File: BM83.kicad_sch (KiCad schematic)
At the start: 41 parts, among them J101 Jack-DC, J102 AudioJack3, J103 USB_C_Receptacle_USB2.0, J104 Conn_01x02, J105 Conn_01x02, SW101 SW_Slide_DPDT, U101 USBLC6-2SC6, U102 CH221K

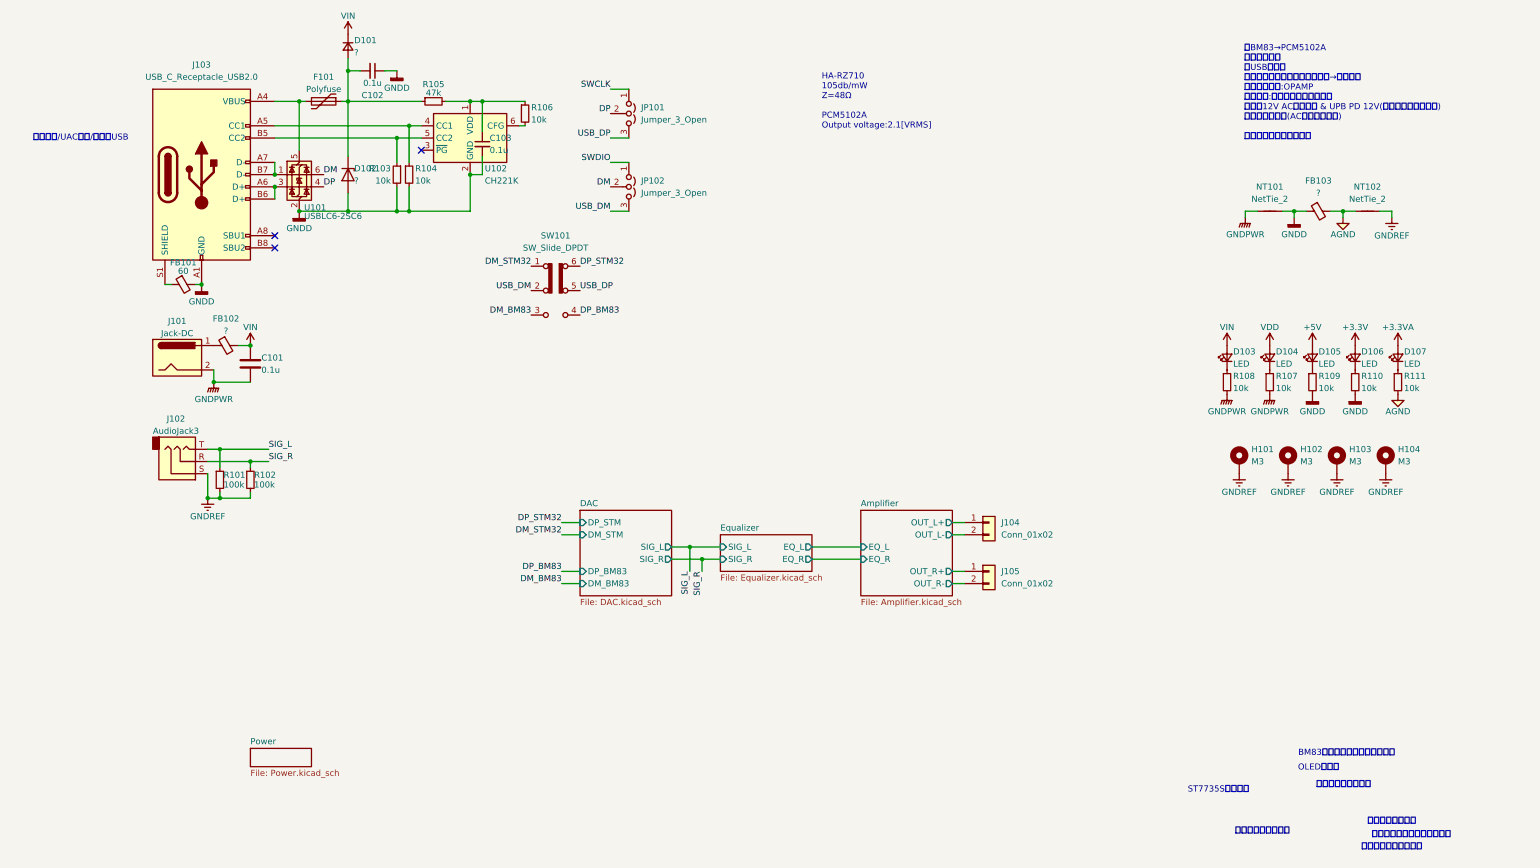
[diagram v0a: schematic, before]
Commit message: 回路図ひとまず完成
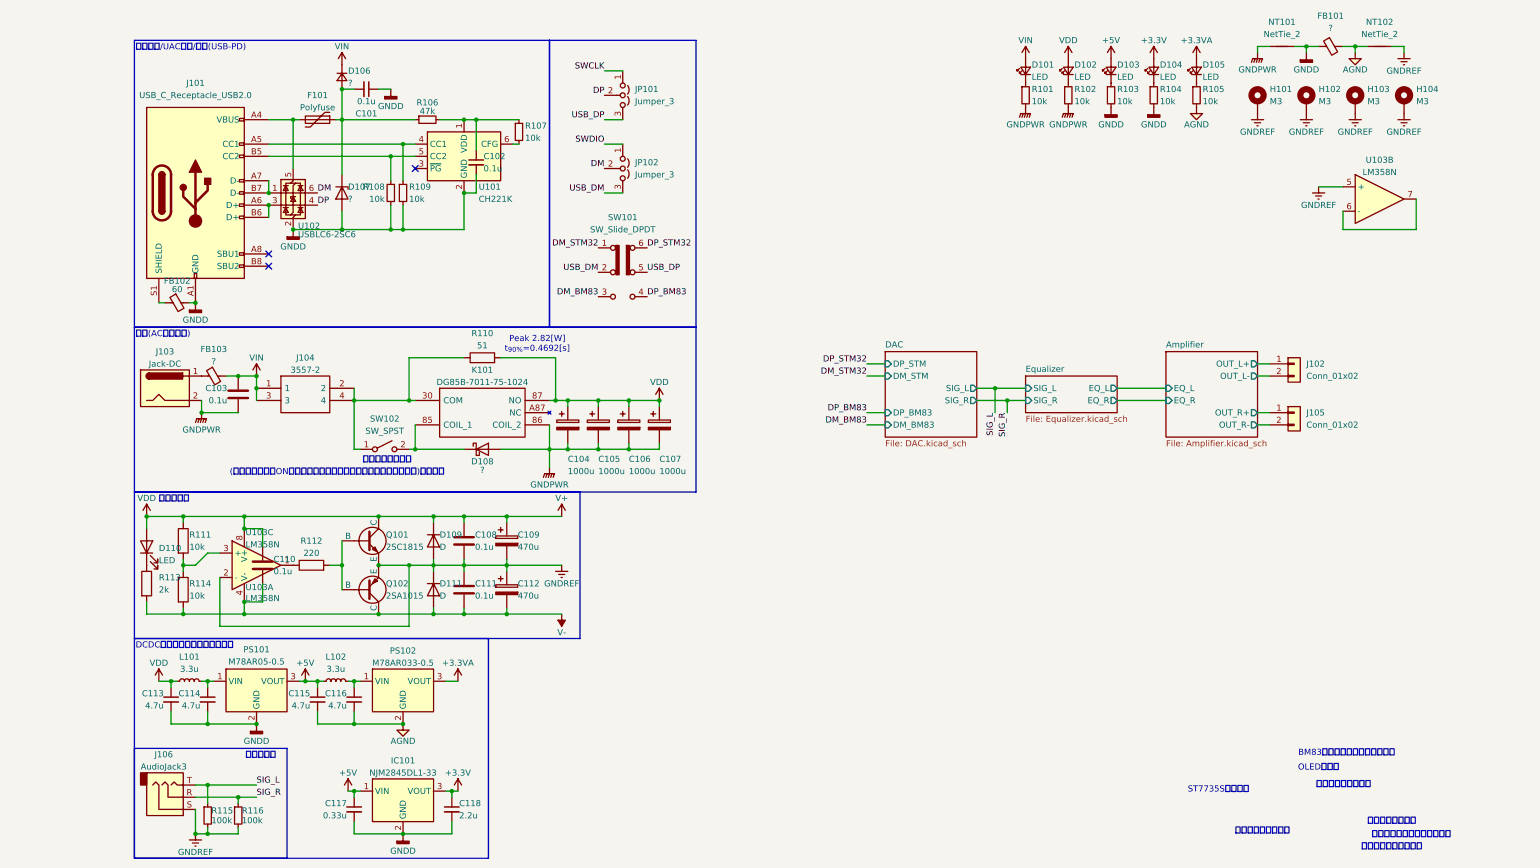
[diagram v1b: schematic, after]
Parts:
- added C104, C105, C106, C107: 1000u, Capacitor_THT:CP_Radial_D16.0mm_P7.50mm, symbol Device:C_Polarized
- added C108, C111: 0.1u, symbol Device:C
- added C109, C112: 470u, Capacitor_THT:CP_Radial_D16.0mm_P7.50mm, symbol Device:C_Polarized
- added C110: 0.1u, Capacitor_THT:C_Disc_D5.1mm_W3.2mm_P5.00mm, symbol Device:C
- added C113, C114, C115, C116: 4.7u, symbol Device:C_Small
- added C117: 0.33u, symbol Device:C_Small
- added C118: 2.2u, symbol Device:C_Small
- added D108: ?, samacsys:CUHS20F30H3F, symbol Device:D_Schottky
- added D109, D111: D, Diode_THT:D_DO-35_SOD27_P7.62mm_Horizontal, symbol Device:D
- added D110: LED, LED_THT:LED_D3.0mm_Horizontal_O1.27mm_Z2.0mm, symbol Device:LED
- added IC101: NJM2845DL1-33, TO-252-3-L1, symbol SamacSys_Parts:NJM2845DL1-33-TE1
- added J104: 3557-2, samacsys:3557-2, symbol SamacSys_Parts:3557-2
- added K101: DG85B-7011-75-1024, MyLibrary:DG85B-7011-75-1024, symbol SamaSys_Parts:DG85B-7011-75-1024
- added L101, L102: 3.3u, symbol Device:L_Small
- added PS101: M78AR05-0.5, M78AR03305, symbol SamacSys_Parts:M78AR05-0.5
- added PS102: M78AR033-0.5, M78AR03305, symbol SamacSys_Parts:M78AR033-0.5
- added Q101: 2SC1815, Package_TO_SOT_THT:TO-92L_Inline_Wide, symbol Simulation_SPICE:NPN
- added Q102: 2SA1015, Package_TO_SOT_THT:TO-92L_Inline_Wide, symbol Simulation_SPICE:PNP
- added R110: 51, symbol Device:R
- added R111, R114: 10k, Resistor_THT:R_Axial_DIN0204_L3.6mm_D1.6mm_P5.08mm_Horizontal, symbol Device:R
- added R112: 220, Resistor_THT:R_Axial_DIN0204_L3.6mm_D1.6mm_P5.08mm_Horizontal, symbol Device:R
- added R113: 2k, Resistor_THT:R_Axial_DIN0204_L3.6mm_D1.6mm_P5.08mm_Horizontal, symbol Device:R
- added SW102: SW_SPST, symbol Switch:SW_SPST
- added U103: LM358N, Package_DIP:DIP-8_W7.62mm_Socket, symbol Device:Opamp_Dual
- JP101, JP102: value Jumper_3_Open -> Jumper_3
- renumbered C102 to C101, C103 to C102, C101 to C103, D103 to D101, D104 to D102, D105 to D103, D106 to D104, D107 to D105, D101 to D106, D102 to D107, FB103 to FB101, FB101 to FB102, FB102 to FB103, J103 to J101, J104 to J102, J101 to J103, J102 to J106, R108 to R101, R107 to R102, R109 to R103, R110 to R104, R111 to R105, R105 to R106, R106 to R107, R103 to R108, R104 to R109, R101 to R115, R102 to R116, U102 to U101, U101 to U102
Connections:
- net +3.3V: now also C118.1, IC101.3 (VOUT)
- net +3.3VA: now also PS102.3 (VOUT)
- net +5V: now also C115.1, C117.1, IC101.1 (VIN), L102.1, PS101.3 (VOUT)
- net AGND: now also C115.2, C116.2, PS102.2 (GND)
- net GNDD: now also C113.2, C114.2, C117.2, C118.2, IC101.2 (GND), PS101.2 (GND)
- net GNDPWR: now also C104.2, C105.2, C106.2, C107.2, D108.2 (A), K101.86 (COIL_2)
- net GNDREF: now also C108.2, C109.2, C111.1, C112.1, D109.2 (A), D111.1 (K), Q101.3 (E), Q102.3 (E), U103.2 (-), U103.5 (+)
- net VIN: now also J104.1, J104.3
- net VDD renamed V+
- net V+: now also C104.1, C105.1, C106.1, C107.1, C108.1, C109.1, C110.1, C113.1, D109.1 (K), D110.2 (A), K101.87 (NO), L101.1, Q101.1 (C), R110.2, R111.1, U103.8 (V+)
- new net: J104.2, J104.4, K101.30 (COM), R110.1, SW102.1 (A)
- new net: Q101.2 (B), Q102.2 (B), R112.2
- new net: D108.1 (K), K101.85 (COIL_1), SW102.2 (B)
- new net: R111.2, R114.1, U103.3 (+)
- new net: C114.1, L101.2, PS101.1 (VIN)
- new net: D110.1 (K), R113.1
- new net: C116.1, L102.2, PS102.1 (VIN)
- new net: R112.1, U103.1
- new net: U103.6 (-), U103.7
- new net V-: C110.2, C111.2, C112.2, D111.2 (A), Q102.1 (C), R113.2, R114.2, U103.4 (V-)
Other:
- removed sheet Power
- note added: "(このスイッチをONした状態で電源接続した際のフールプルーフは)ないです"
- note added: "DCDCコンバータ・レギュレータ"
- note added: "Peak 2.82[W] t_{90%}=0.4692[s]"
- note added: "ミサイルスイッチ"
- note added: "ライン入力"
- note added: "両電源生成"
- note added: "書き込み/UAC接続/給電(USB-PD)"
- note added: "給電(ACアダプタ)"
- note removed: "HA-RZ710 105db/mW Z=48Ω PCM5102A Output voltage:2.1[VRMS]"
- note removed: "・BM83→PCM5102A ・ライン入力 ・USB入力？ これらの後段でシングルエンド→差動変換 ・電圧増幅段:OPAMP ・出力段:ダイヤモンドバッファ ・電源12V ACアダプタ & UPB PD 12V(差動である点に留意) ・電源優先回路(ACアダプタ優先) 数値要件は手元の紙参照"
- note removed: "書き込み/UAC接続/給電用USB"
- moved on the sheet: C101, C102, C103, D101, D102, D103, D104, D105, D106, D107, F101, FB101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
